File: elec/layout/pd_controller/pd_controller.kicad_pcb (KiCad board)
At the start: 2 copper layers, 26.4 x 17.6 mm, 17 parts, among them Q1 MOSFET, U1 STUSB4500QTR

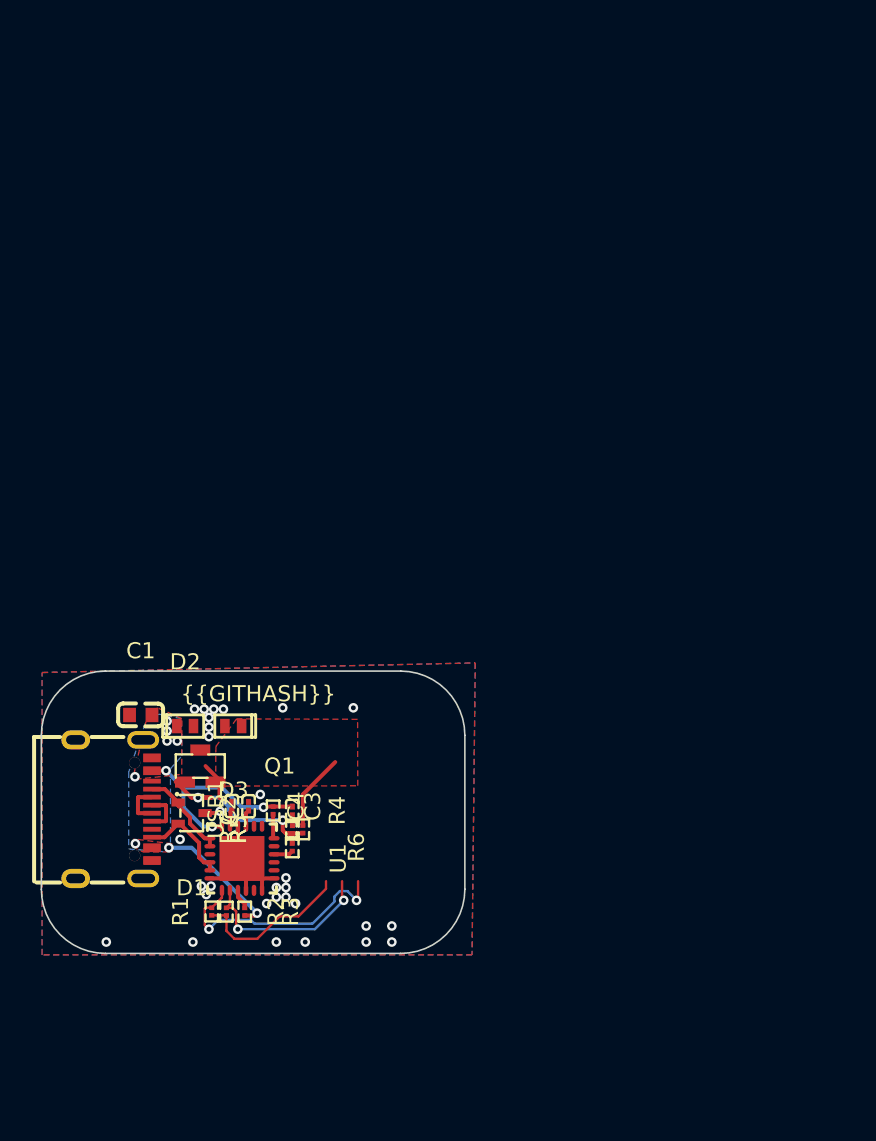
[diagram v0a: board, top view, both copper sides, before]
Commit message: layout 95%
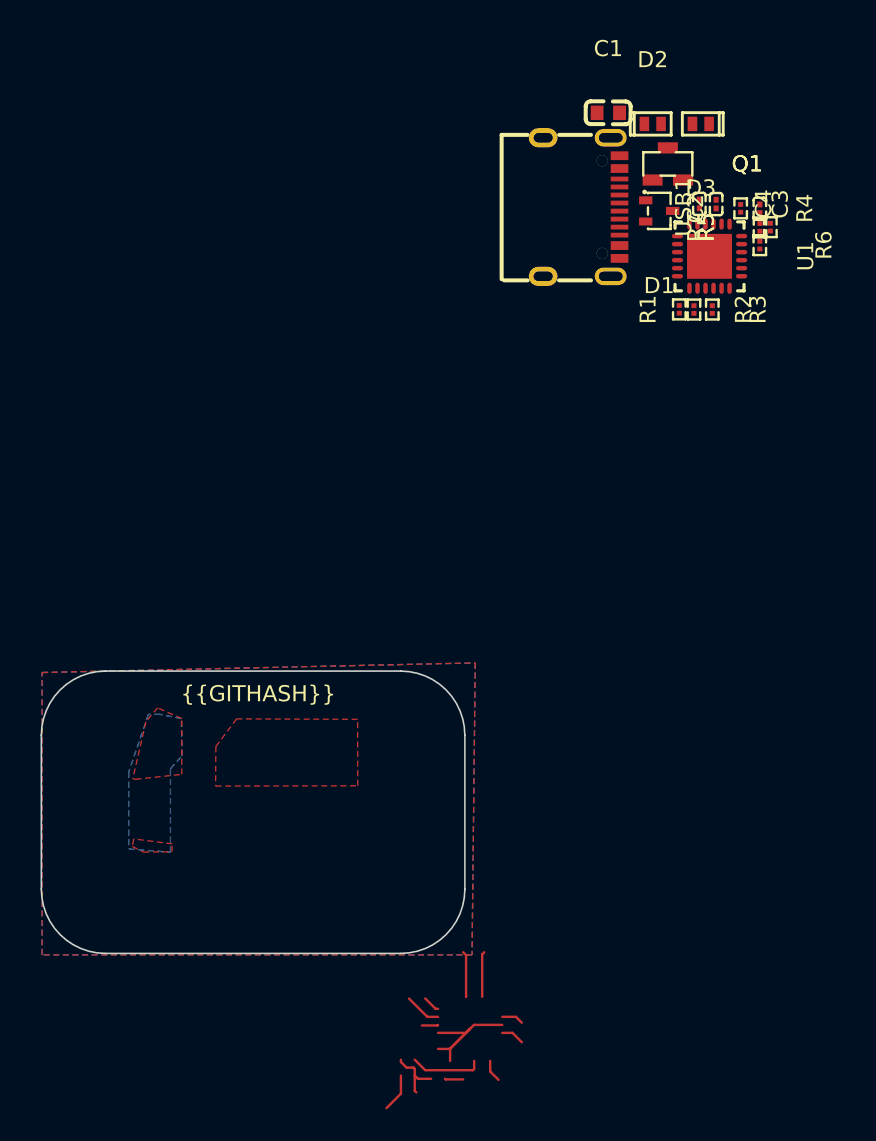
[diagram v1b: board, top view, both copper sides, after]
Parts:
- moved Q1 47.5 mm to (168.4, 57.5)
- moved R2 47.5 mm to (169.1, 66.6)
- moved R7 47.5 mm to (174.1, 61.5)
- moved U1 47.5 mm to (171.0, 63.2)
- moved C1 47.5 mm to (164.7, 54.3)
- moved C2 47.5 mm to (174.1, 60.3)
- moved D1 47.5 mm to (167.9, 60.4)
- moved R6 47.5 mm to (174.1, 62.6)
- moved USB1 47.5 mm to (163.0, 60.2)
- moved R1 47.5 mm to (171.2, 66.6)
- moved C3 47.5 mm to (171.4, 60.0)
- moved C4 47.5 mm to (170.4, 60.0)
- moved D2 47.5 mm to (167.5, 55.0)
- moved D3 47.5 mm to (170.5, 55.0)
- moved R4 47.5 mm to (172.9, 60.3)
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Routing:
- net VBUS: track 22.2 -> 0.00 mm, vias 11 -> 0
- net (no net): track 22.2 -> 0.00 mm, vias 2 -> 0
- net I2C_SCL: track 15.2 -> 0.00 mm, vias 2 -> 0
- net lv: track 12.7 -> 0.00 mm, vias 30 -> 0
- net I2C_SDA: track 11.6 -> 0.00 mm, vias 2 -> 0
- net 32: track 0.00 -> 9.23 mm
- net VSINK_VCC: track 7.14 -> 0.00 mm
- net CC2: track 5.99 -> 0.00 mm
- net CC1: track 5.72 -> 0.00 mm
- net 36: track 0.00 -> 4.51 mm
- net 31: track 0.00 -> 3.80 mm
- net 27: track 0.00 -> 2.86 mm
- net 28: track 0.00 -> 2.83 mm
- net USB_CONNECTOR-net-1: track 2.72 -> 0.00 mm
- net USB_CONNECTOR-net: track 2.72 -> 0.00 mm
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
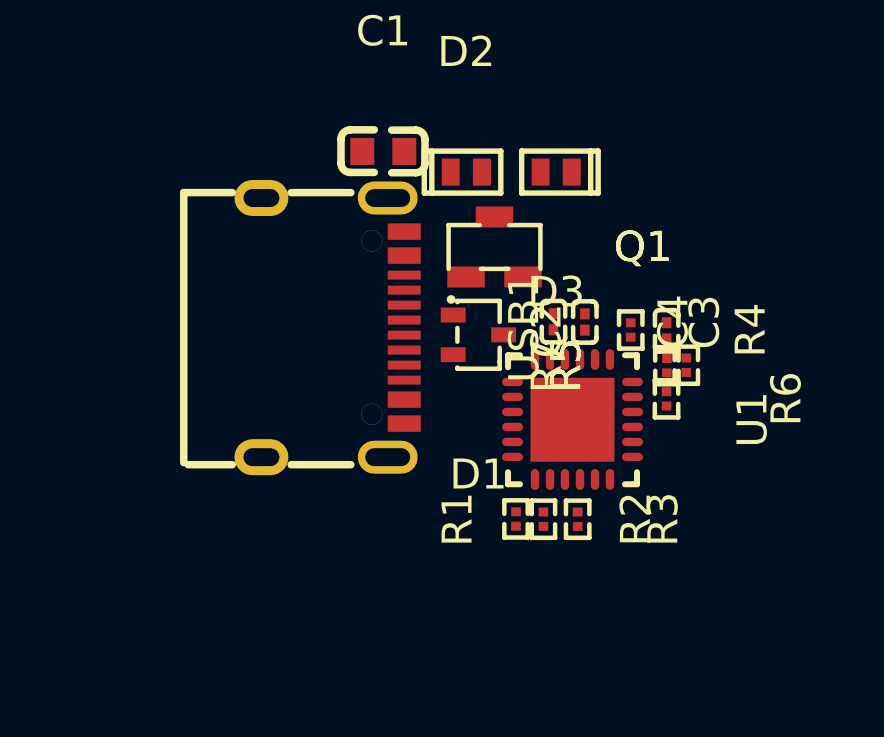
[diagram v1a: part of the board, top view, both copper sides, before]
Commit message: Build full
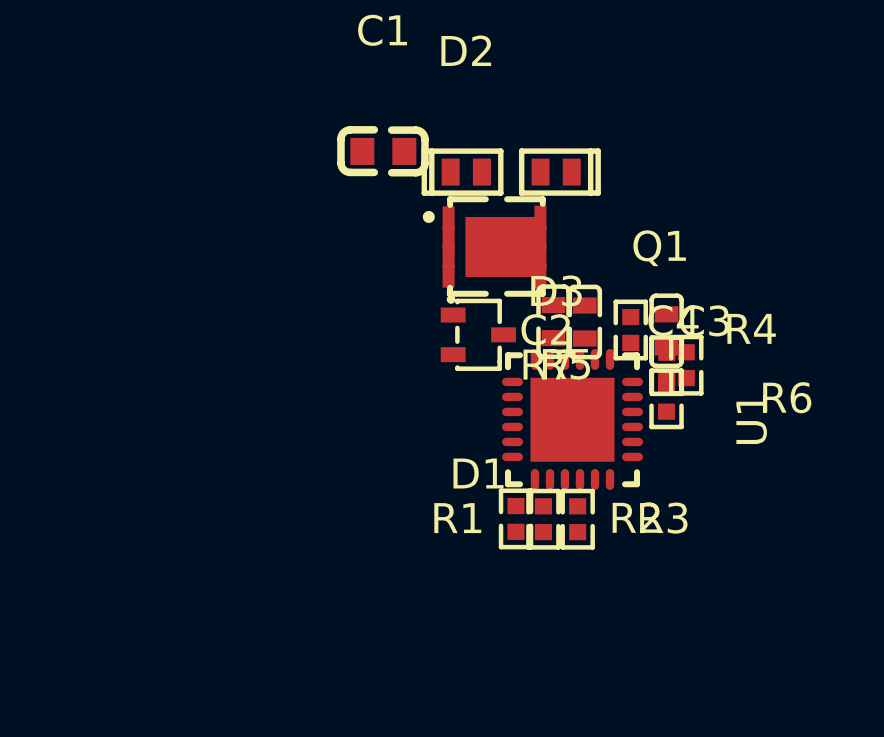
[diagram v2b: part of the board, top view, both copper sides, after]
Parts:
- removed USB1: TYPE_C_16PIN_2MD073, lcsc:USB-C-SMD_TYPE-C-6PIN-2MD-073
- C2: value 100nF ±10% 10V X5R -> 1µF ±10% 10V X5R; footprint lcsc:C0201 -> lcsc:C0402
- C3: value 1µF ±20% 6.3V X5R -> 1µF ±10% 10V X5R; footprint lcsc:C0201 -> lcsc:C0402
- C4: value (none) -> 100nF ±10% 16V X7R; footprint lcsc:C0201 -> lcsc:C0402
- D2, D3: value (none) -> infV
- Q1: footprint lcsc:SOT-23-3_L2.9-W1.3-P1.90-LS2.4-BR -> lcsc:PDFN3333-8_L3.1-W3.2-P0.65-LS3.4-BL
- R1: value 1kΩ ±1% 50mW -> 1kΩ ±1% 62.5mW; footprint lcsc:R0201 -> lcsc:R0402
- R2: value 4.64kΩ ±1% 50mW -> 4.7kΩ ±1% 62.5mW; footprint lcsc:R0201 -> lcsc:R0402
- R3: value (none) -> 4.7kΩ ±1% 62.5mW; footprint lcsc:R0201 -> lcsc:R0402
- R4: value (none) -> 1kΩ ±1% 62.5mW; footprint lcsc:R0201 -> lcsc:R0402
- R5: value 100kΩ ±1% 50mW -> 100kΩ ±1% 62.5mW; footprint lcsc:R0201 -> lcsc:R0402
- R6: value 22.1kΩ ±1% 50mW -> 22kΩ ±1% 62.5mW; footprint lcsc:R0201 -> lcsc:R0402
- R7: value 100Ω ±1% 50mW -> 100Ω ±1% 62.5mW; footprint lcsc:R0201 -> lcsc:R0402
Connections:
- net I2C_SCL renamed signal-1
- net I2C_SDA renamed signal
- net PD_CONTROLLER.footprint.pins[18].net-net renamed pd_controller.footprint.pins[18].net-net
- C2 pad 1: net-4 -> lv
- C2 pad 2: VBUS -> VREG_1V2
- C3 pad 2: VREG_1V2 -> VREG_2V7
- C4 pad 1: lv -> net-3
- C4 pad 2: VREG_2V7 -> VBUS
- Q1 pad 1: net-3 -> VBUS
- Q1 pad 3: VSINK_VCC -> VBUS
- R1 pad 2: net-1 -> net-4
- R5 pad 1: net-3 -> net
- R6 pad 1: net-3 -> net
- R6 pad 2: net -> net-1
- R7 pad 1: net-3 -> net
- R7 pad 2: net-4 -> net-3
- U1 pad 1: CC1 -> pd_controller-signal-1
- U1 pad 16: net -> net-1
- U1 pad 5: CC2 -> pd_controller-signal
- U1 pad 9: net-1 -> net-4
